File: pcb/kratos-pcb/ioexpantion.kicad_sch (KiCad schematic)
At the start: 7 parts, among them IC2 SN74HC595N, J2 Screw_Terminal_01x04, J3 Screw_Terminal_01x04, U2 ULN2803A, U3 ULN2803A

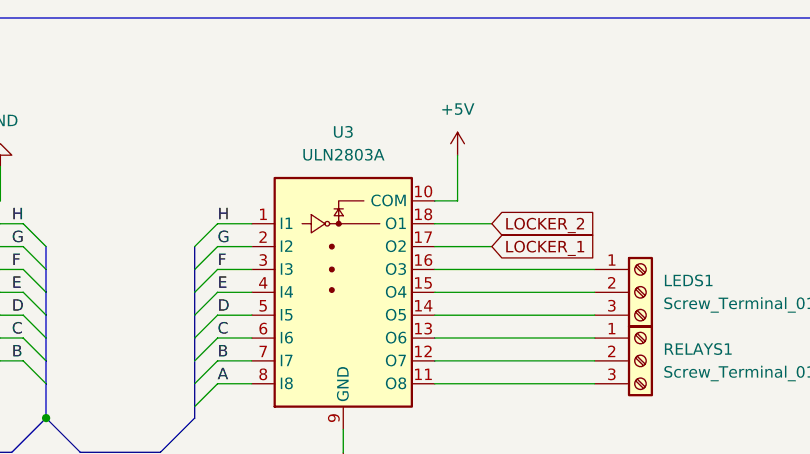
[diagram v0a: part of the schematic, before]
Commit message: ### MODIFY
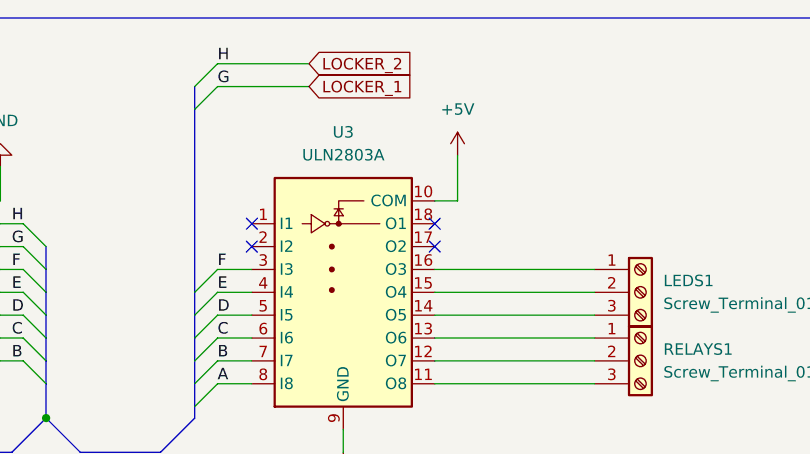
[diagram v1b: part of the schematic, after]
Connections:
- net LOCKER_1: now also IC2.6 (QG); no longer U3.17 (O2)
- net LOCKER_2: now also IC2.7 (QH_1); no longer U3.18 (O1)
- net G: no longer names the net of U3.2 (I2)
- net G: no longer IC2.6 (QG)
- net H: no longer names the net of U3.1 (I1)
- net H: no longer IC2.7 (QH_1)
- no-connect marks 3 -> 7
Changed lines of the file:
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@@
   )
   (no_connect (at 71.12 139.7))
+  (no_connect (at 133.35 64.77))
   (no_connect (at 54.61 59.69))
+  (no_connect (at 113.03 62.23))
+  (no_connect (at 133.35 62.23))
   (no_connect (at 91.44 139.7))
+  (no_connect (at 113.03 64.77))
   (bus_entry (at 87.63 72.39) (size 2.54 2.54)
     (stroke (width 0) (type default))
@@
     (stroke (width 0) (type default))
   )
-  (bus_entry (at 109.22 62.23) (size -2.54 2.54)
+  (bus_entry (at 109.22 44.45) (size -2.54 2.54)
     (stroke (width 0) (type default))
   )
@@
     (stroke (width 0) (type default))
   )
-  (bus_entry (at 109.22 64.77) (size -2.54 2.54)
+  (bus_entry (at 109.22 46.99) (size -2.54 2.54)
     (stroke (width 0) (type default))
   )
@@
     (stroke (width 0) (type default))
   )
-  (bus (pts (xy 106.68 67.31) (xy 106.68 69.85))
+  (bus (pts (xy 106.68 49.53) (xy 106.68 69.85))
     (stroke (width 0) (type default))
   )
@@
     (stroke (width 0) (type default))
   )
-  (wire (pts (xy 133.35 62.23) (xy 139.7 62.23))
-    (stroke (width 0) (type default))
-  )
   (wire (pts (xy 135.89 54.61) (xy 135.89 59.69))
     (stroke (width 0) (type default))
@@
     (stroke (width 0) (type default))
   )
-  (wire (pts (xy 109.22 62.23) (xy 113.03 62.23))
-    (stroke (width 0) (type default))
-  )
   (wire (pts (xy 85.09 77.47) (xy 87.63 77.47))
     (stroke (width 0) (type default))
@@
     (stroke (width 0) (type default))
   )
-  (bus (pts (xy 106.68 64.77) (xy 106.68 67.31))
+  (bus (pts (xy 106.68 46.99) (xy 106.68 49.53))
     (stroke (width 0) (type default))
   )
@@
     (stroke (width 0) (type default))
   )
-  (wire (pts (xy 133.35 64.77) (xy 139.7 64.77))
+  (wire (pts (xy 109.22 44.45) (xy 119.38 44.45))
     (stroke (width 0) (type default))
   )
@@
     (stroke (width 0) (type default))
   )
-  (wire (pts (xy 109.22 64.77) (xy 113.03 64.77))
+  (wire (pts (xy 109.22 46.99) (xy 119.38 46.99))
     (stroke (width 0) (type default))
   )
@@
     (effects (font (size 1.27 1.27)) (justify left bottom))
   )
-  (label "H" (at 109.22 62.23 0) (fields_autoplaced)
+  (label "H" (at 109.22 44.45 0) (fields_autoplaced)
     (effects (font (size 1.27 1.27)) (justify left bottom))
   )
@@
     (effects (font (size 1.27 1.27)) (justify left bottom))
   )
-  (label "G" (at 109.22 64.77 0) (fields_autoplaced)
+  (label "G" (at 109.22 46.99 0) (fields_autoplaced)
     (effects (font (size 1.27 1.27)) (justify left bottom))
   )
@@
     )
   )
-  (global_label "LOCKER_1" (shape input) (at 139.7 64.77 0) (fields_autoplaced)
+  (global_label "LOCKER_2" (shape input) (at 119.38 44.45 0) (fields_autoplaced)
     (effects (font (size 1.27 1.27)) (justify left))
-    (property "Intersheetrefs" "${INTERSHEET_REFS}" (at 152.1799 64.77 0)
+    (property "Intersheetrefs" "${INTERSHEET_REFS}" (at 131.8599 44.45 0)
       (effects (font (size 1.27 1.27)) (justify left) hide)
     )
@@
     )
   )
-  (global_label "LOCKER_2" (shape input) (at 139.7 62.23 0) (fields_autoplaced)
+  (global_label "BLUE-LED-2" (shape input) (at 67.31 137.16 180) (fields_autoplaced)
+    (effects (font (size 1.27 1.27)) (justify right))
+    (property "Intersheetrefs" "${INTERSHEET_REFS}" (at 51.7458 137.16 0)
+      (effects (font (size 1.27 1.27)) (justify right) hide)
+    )
+  )
+  (global_label "GREEN-LED" (shape input) (at 67.31 127 180) (fields_autoplaced)
+    (effects (font (size 1.27 1.27)) (justify right))
+    (property "Intersheetrefs" "${INTERSHEET_REFS}" (at 53.1368 127 0)
+      (effects (font (size 1.27 1.27)) (justify right) hide)
+    )
+  )
+  (global_label "BLUE-LED" (shape input) (at 67.31 129.54 180) (fields_autoplaced)
+    (effects (font (size 1.27 1.27)) (justify right))
+    (property "Intersheetrefs" "${INTERSHEET_REFS}" (at 54.5277 129.54 0)
+      (effects (font (size 1.27 1.27)) (justify right) hide)
+    )
+  )
+  (global_label "RED-LED" (shape input) (at 67.31 124.46 180) (fields_autoplaced)
+    (effects (font (size 1.27 1.27)) (justify right))
+    (property "Intersheetrefs" "${INTERSHEET_REFS}" (at 55.6163 124.46 0)
+      (effects (font (size 1.27 1.27)) (justify right) hide)
+    )
+  )
+  (global_label "GREEN-LED-2" (shape input) (at 67.31 134.62 180) (fields_autoplaced)
+    (effects (font (size 1.27 1.27)) (justify right))
+    (property "Intersheetrefs" "${INTERSHEET_REFS}" (at 50.3549 134.62 0)
+      (effects (font (size 1.27 1.27)) (justify right) hide)
+    )
+  )
+  (global_label "LOCKER_1" (shape input) (at 119.38 46.99 0) (fields_autoplaced)
     (effects (font (size 1.27 1.27)) (justify left))
-    (property "Intersheetrefs" "${INTERSHEET_REFS}" (at 152.1799 62.23 0)
+    (property "Intersheetrefs" "${INTERSHEET_REFS}" (at 131.8599 46.99 0)
       (effects (font (size 1.27 1.27)) (justify left) hide)
     )
   )
-  (global_label "BLUE-LED-2" (shape input) (at 67.31 137.16 180) (fields_autoplaced)
-    (effects (font (size 1.27 1.27)) (justify right))
-    (property "Intersheetrefs" "${INTERSHEET_REFS}" (at 51.7458 137.16 0)
-      (effects (font (size 1.27 1.27)) (justify right) hide)
-    )
-  )
-  (global_label "GREEN-LED" (shape input) (at 67.31 127 180) (fields_autoplaced)
-    (effects (font (size 1.27 1.27)) (justify right))
-    (property "Intersheetrefs" "${INTERSHEET_REFS}" (at 53.1368 127 0)
-      (effects (font (size 1.27 1.27)) (justify right) hide)
-    )
-  )
-  (global_label "BLUE-LED" (shape input) (at 67.31 129.54 180) (fields_autoplaced)
-    (effects (font (size 1.27 1.27)) (justify right))
-    (property "Intersheetrefs" "${INTERSHEET_REFS}" (at 54.5277 129.54 0)
-      (effects (font (size 1.27 1.27)) (justify right) hide)
-    )
-  )
-  (global_label "RED-LED" (shape input) (at 67.31 124.46 180) (fields_autoplaced)
-    (effects (font (size 1.27 1.27)) (justify right))
-    (property "Intersheetrefs" "${INTERSHEET_REFS}" (at 55.6163 124.46 0)
-      (effects (font (size 1.27 1.27)) (justify right) hide)
-    )
-  )
-  (global_label "GREEN-LED-2" (shape input) (at 67.31 134.62 180) (fields_autoplaced)
-    (effects (font (size 1.27 1.27)) (justify right))
-    (property "Intersheetrefs" "${INTERSHEET_REFS}" (at 50.3549 134.62 0)
-      (effects (font (size 1.27 1.27)) (justify right) hide)
-    )
-  )
